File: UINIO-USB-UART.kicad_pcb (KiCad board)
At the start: 2 copper layers, 72.2 x 20.5 mm, 34 parts, among them J1 Conn_01x08_Male, J2 Conn_01x04_Male, J3 Conn_01x07_Male, J4 Conn_01x06_Male, J5 Conn_01x04_Male, J6 Conn_01x07_Male, SW1 TP-33103, U1 CP2102, U2 CH343P

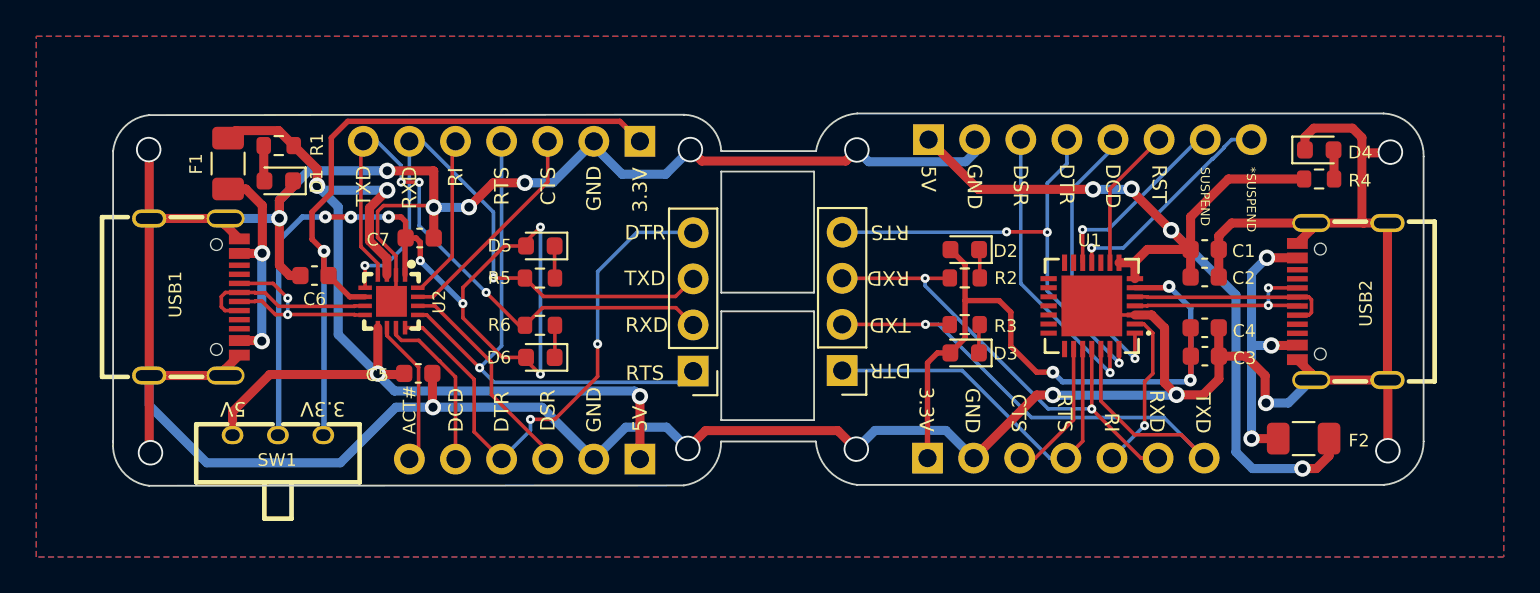
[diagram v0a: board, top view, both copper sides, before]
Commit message: Update README.md.
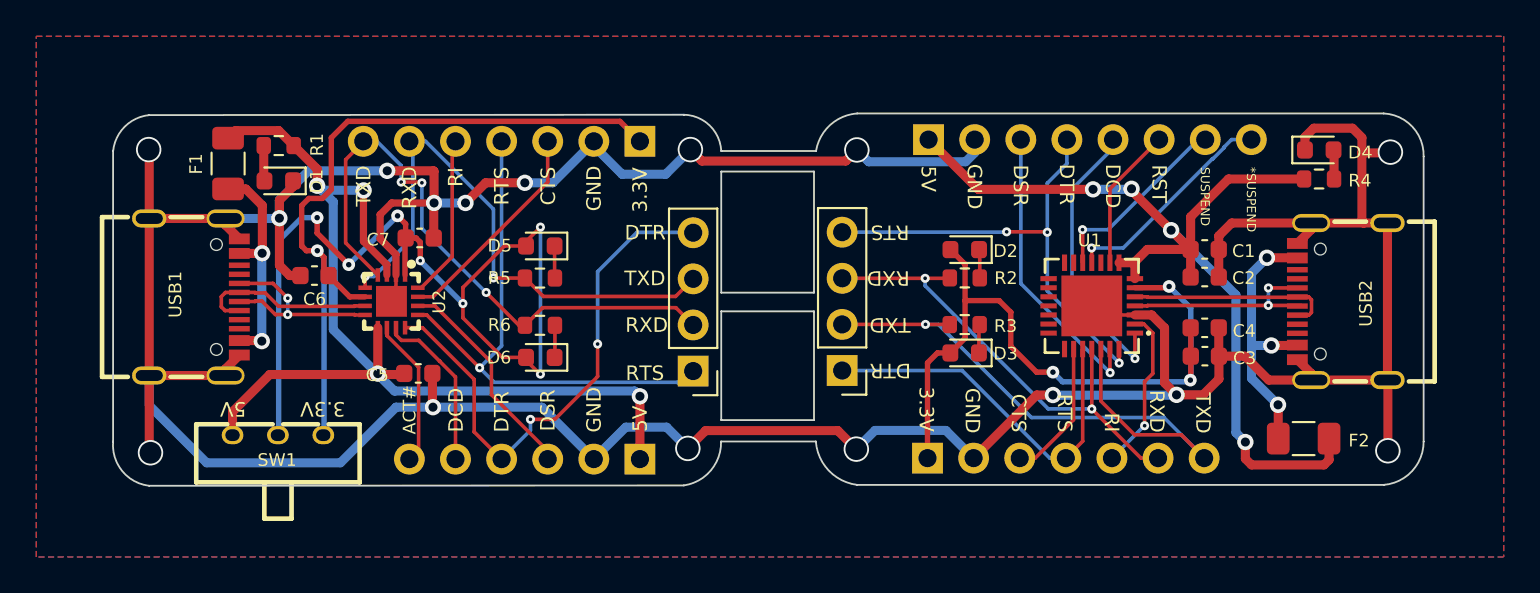
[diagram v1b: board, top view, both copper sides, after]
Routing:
- net GND: track 228.1 -> 224.2 mm, vias 17 -> 16
- net /CH343_VIO: track 47.4 -> 50.0 mm
- net /CH343_VDD_5V: track 60.6 -> 59.0 mm
- net /CH343_VDD_3.3V: track 38.6 -> 40.0 mm
- net Net-(USB2-PadA4B9): track 16.0 -> 15.1 mm
- net /CH343_TXD: track 32.9 -> 33.7 mm

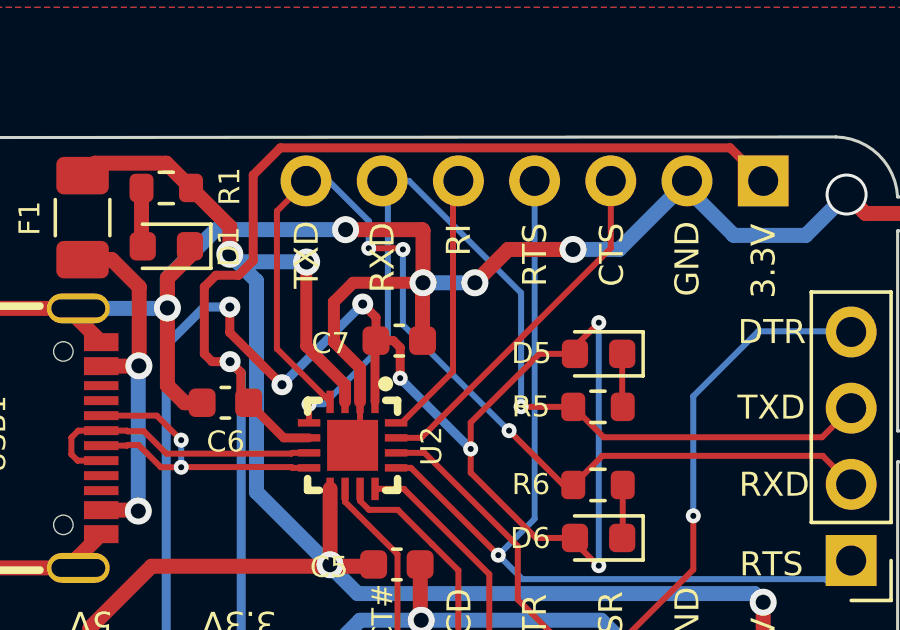
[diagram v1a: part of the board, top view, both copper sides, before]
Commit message: Update README.md.
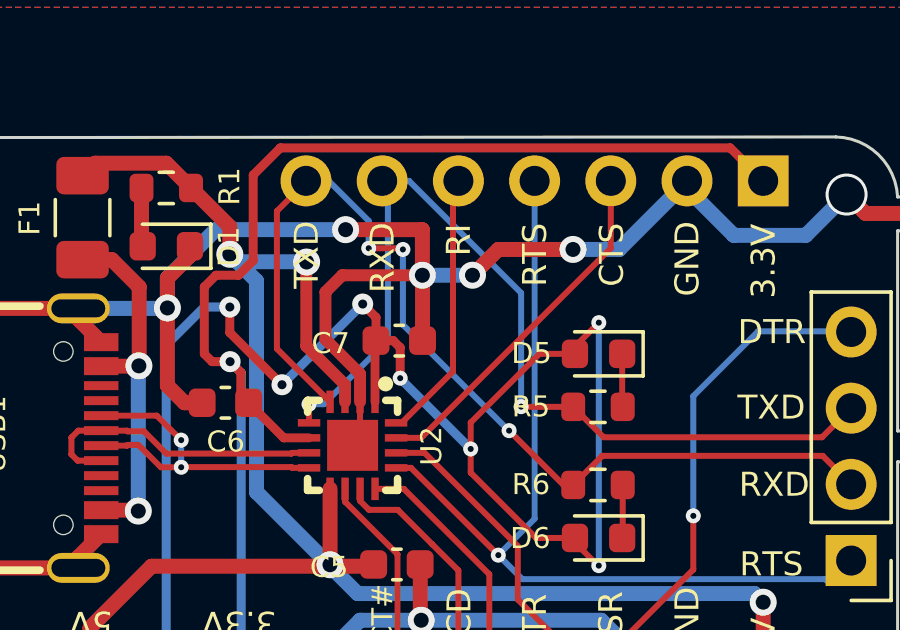
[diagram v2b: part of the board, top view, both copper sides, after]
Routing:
- net GND: track 224.2 -> 224.8 mm
